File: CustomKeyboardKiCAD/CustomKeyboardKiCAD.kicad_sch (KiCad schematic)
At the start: 59 parts, among them J1 USB_C_Receptacle_USB2.0_16P, J2 Display Connector, J3 S2B-PH-K-SLFSN, J4 Conn_01x12, J5 Conn_01x12, SW91 RotaryEncoder_Switch, U1 nRF52840, U2 XC6220B331MR, U3 74HC595, U4 BQ24075RGTR, U5 74HC595, U6 74HC595, U7 nice_nano, Y1 32.768kHz FC-12M, Y2 32MHz XRCGB32MOODF1H5ORO

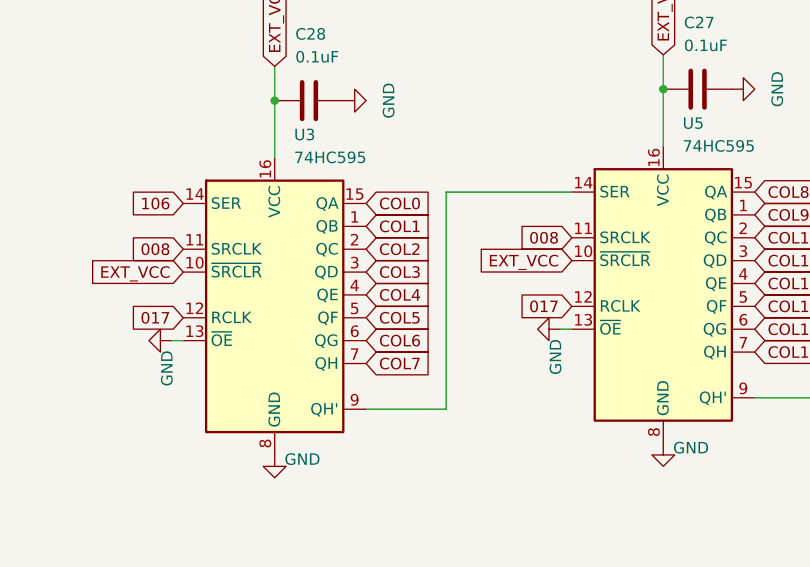
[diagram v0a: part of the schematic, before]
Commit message: more progress on pcb
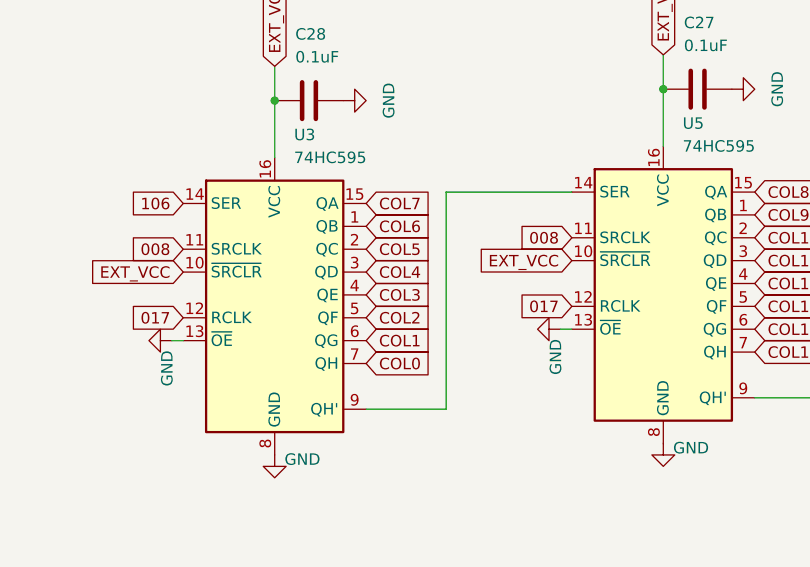
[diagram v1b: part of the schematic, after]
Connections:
- net COL0: now also U3.7 (QH); no longer U3.15 (QA)
- net COL1: now also U3.6 (QG); no longer U3.1 (QB)
- net COL2: now also U3.5 (QF); no longer U3.2 (QC)
- net COL3: now also U3.4 (QE); no longer U3.3 (QD)
- net COL4: now also U3.3 (QD); no longer U3.4 (QE)
- net COL5: now also U3.2 (QC); no longer U3.5 (QF)
- net COL6: now also U3.1 (QB); no longer U3.6 (QG)
- net COL7: now also U3.15 (QA); no longer U3.7 (QH)
